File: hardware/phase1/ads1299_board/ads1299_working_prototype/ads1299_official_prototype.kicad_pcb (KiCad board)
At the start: 4 copper layers, 101.5 x 94 mm, 106 parts, among them J2 1725656, J3 TSM-110-01-T-DV-P-TR, J5 TSW-103-07-T-D, J6 36PIN_IDC, J9 1725656, U1 ADS1299IPAG, U10 24AA256-I/ST, U11 OPA376AID, U4 OPA376

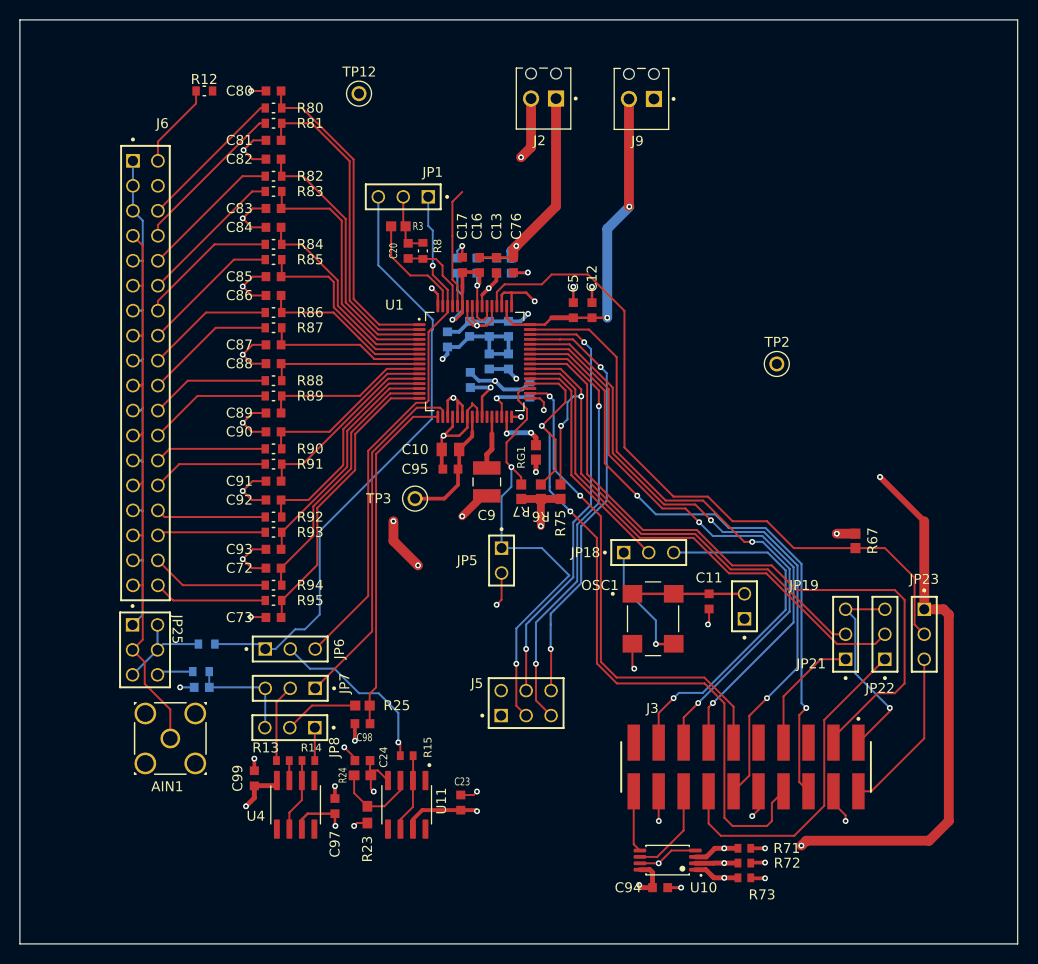
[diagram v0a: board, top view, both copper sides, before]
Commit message: Chat it's done
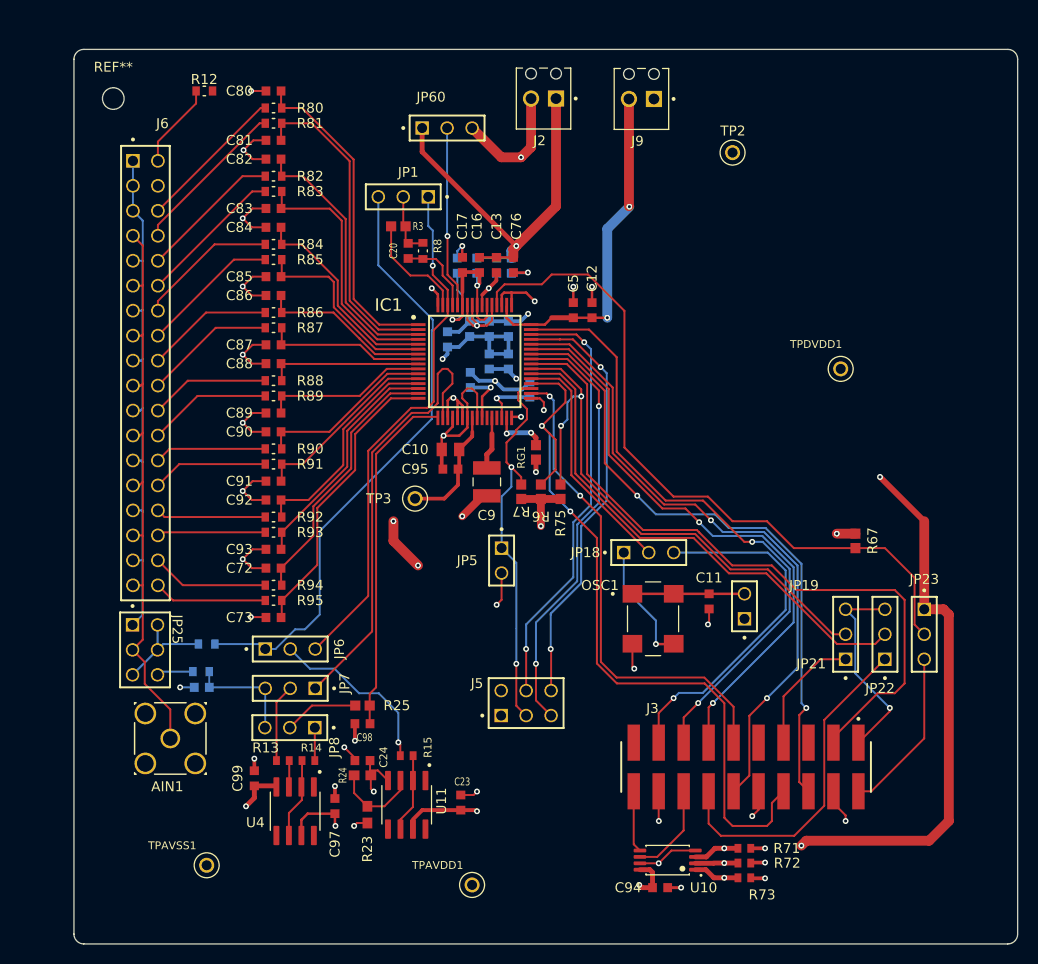
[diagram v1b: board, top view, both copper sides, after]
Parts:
- removed TP12: 5001, 5001:KEYSTONE_5001
- added JP60: TSW-103-07-T-S, TSW-103-07-T-S:SAMTEC_TSW-103-07-T-S, F.Cu at (133.0, 51.0)
- added REF**: MountingHole_2.2mm_M2, MountingHole:MountingHole_2.2mm_M2, F.Cu at (99.0, 48.0)
- added TPAVDD1: AVDD, 5000:KEYSTONE_5000, F.Cu at (135.5, 128.0)
- added TPAVSS1: AVSS, 5000:KEYSTONE_5000, F.Cu at (108.5, 126.0)
- added TPDVDD1: DVDD, 5000:KEYSTONE_5000, F.Cu at (173.0, 75.5)
- IC1: renamed from U1; value ADS1299IPAG -> ADS1299-4PAGR; footprint ADS1299CPAG:QFP64P50_1200X1200X120L60X22N -> KiCad:QFP50P1200X1200X120-64N
- moved TP2 22.0 mm to (162.0, 53.5)
- moved U4 0.65 mm to (117.5, 120.5)
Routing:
- net AVSS: track 186.0 -> 215.4 mm
- net AVDD: track 159.5 -> 174.3 mm
- net DVDD: track 168.4 -> 180.2 mm
- net SRB2: track 36.2 -> 44.9 mm
- net /PWDN: track 46.2 -> 39.3 mm
- net BIASREF: track 12.2 -> 18.5 mm, vias 0 -> 1
- net /RESET: track 79.6 -> 77.3 mm
- net Net-(U4--IN): track 7.50 -> 8.84 mm
- net Net-(U4-+IN): track 2.04 -> 2.69 mm
- net Net-(J3-Pad07): track 13.2 -> 12.6 mm
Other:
- board size 101.5 x 94 mm -> 96 x 91 mm
